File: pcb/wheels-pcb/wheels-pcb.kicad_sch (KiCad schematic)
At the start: 16 parts, among them J1 Motor_1, J2 Motor_2, J3 Motor_3, J4 Motor_4, J5 Conn_01x03, U1 L293D, U2 L293D, U3 ESP32S_38P

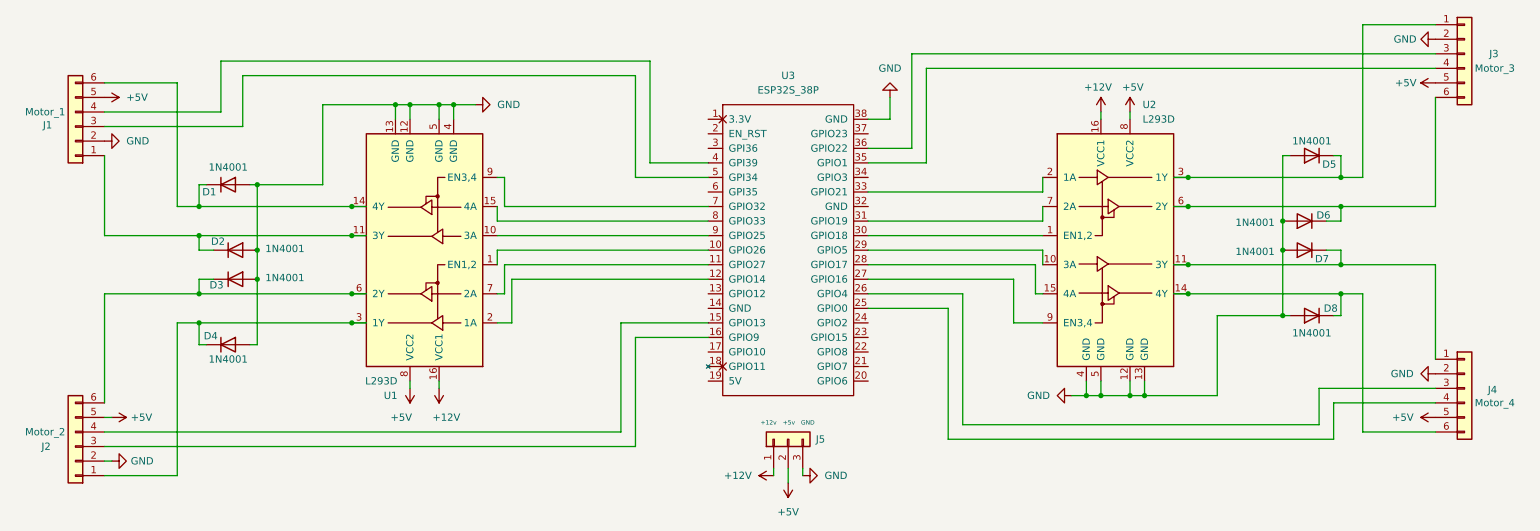
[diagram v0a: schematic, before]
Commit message: pcb correction
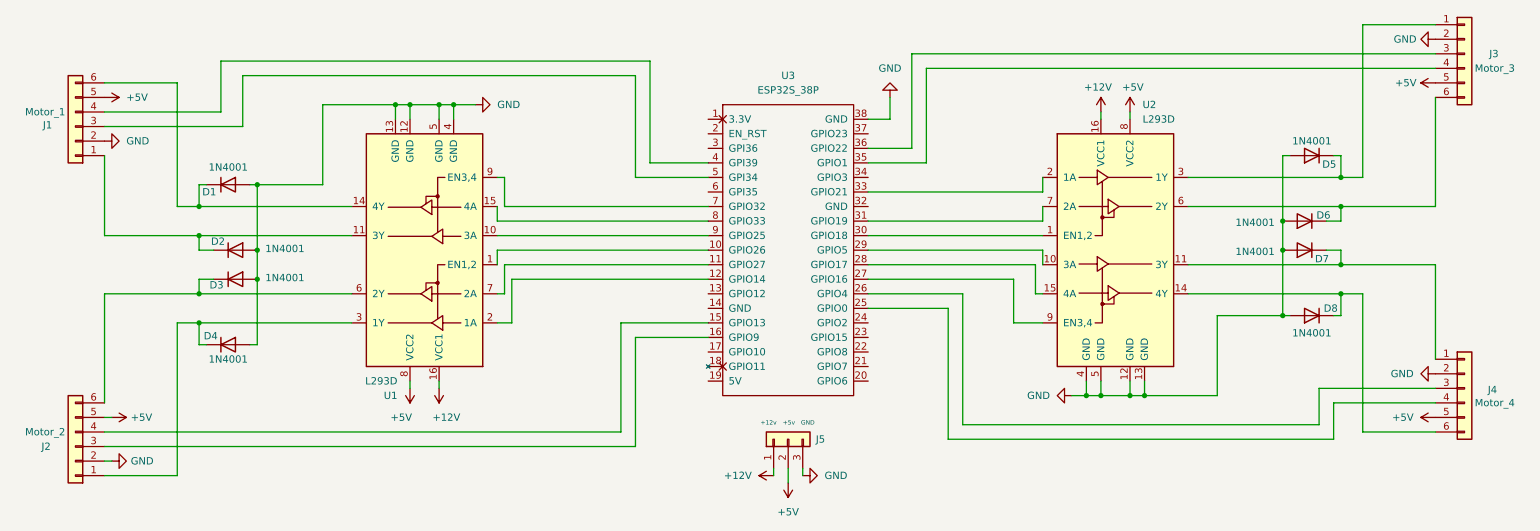
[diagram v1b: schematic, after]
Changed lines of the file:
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@@
-	)
-	(junction
-		(at 222.25 82.55)
-		(diameter 0)
-		(color 0 0 0 0)
 	)
 	(junction
@@
 	)
 	(junction
-		(at 222.25 97.79)
-		(diameter 0)
-		(color 0 0 0 0)
-	)
-	(junction
-		(at 76.2 107.95)
-		(diameter 0)
-		(color 0 0 0 0)
-	)
-	(junction
 		(at 86.36 69.85)
 		(diameter 0)
@@
 	)
 	(junction
-		(at 222.25 102.87)
-		(diameter 0)
-		(color 0 0 0 0)
-	)
-	(junction
-		(at 76.2 92.71)
-		(diameter 0)
-		(color 0 0 0 0)
-	)
-	(junction
 		(at 238.76 95.25)
-		(diameter 0)
-		(color 0 0 0 0)
-	)
-	(junction
-		(at 222.25 87.63)
-		(diameter 0)
-		(color 0 0 0 0)
-	)
-	(junction
-		(at 76.2 102.87)
 		(diameter 0)
 		(color 0 0 0 0)
@@
 	)
 	(junction
-		(at 76.2 87.63)
-		(diameter 0)
-		(color 0 0 0 0)
-	)
-	(junction
 		(at 204.47 120.65)
 		(diameter 0)
@@
 	(wire
 		(pts
-			(xy 78.74 87.63) (xy 76.2 87.63)
-		)
-		(stroke
-			(width 0)
-			(type default)
-		)
-	)
-	(wire
-		(pts
 			(xy 212.09 118.11) (xy 212.09 120.65)
 		)
@@
 	(wire
 		(pts
-			(xy 78.74 107.95) (xy 76.2 107.95)
-		)
-		(stroke
-			(width 0)
-			(type default)
-		)
-	)
-	(wire
-		(pts
 			(xy 248.92 97.79) (xy 265.43 97.79)
 		)
@@
 	(wire
 		(pts
-			(xy 78.74 92.71) (xy 76.2 92.71)
-		)
-		(stroke
-			(width 0)
-			(type default)
-		)
-	)
-	(wire
-		(pts
 			(xy 247.65 106.68) (xy 248.92 106.68)
 		)
@@
 	(wire
 		(pts
-			(xy 219.71 102.87) (xy 222.25 102.87)
-		)
-		(stroke
-			(width 0)
-			(type default)
-		)
-	)
-	(wire
-		(pts
 			(xy 173.99 60.96) (xy 173.99 77.47)
 		)
@@
 	(wire
 		(pts
-			(xy 219.71 82.55) (xy 222.25 82.55)
-		)
-		(stroke
-			(width 0)
-			(type default)
-		)
-	)
-	(wire
-		(pts
 			(xy 182.88 125.73) (xy 245.11 125.73)
 		)
@@
 	(wire
 		(pts
-			(xy 219.71 97.79) (xy 222.25 97.79)
-		)
-		(stroke
-			(width 0)
-			(type default)
-		)
-	)
-	(wire
-		(pts
 			(xy 196.85 97.79) (xy 196.85 95.25)
 		)
@@
 	(wire
 		(pts
-			(xy 219.71 87.63) (xy 222.25 87.63)
-		)
-		(stroke
-			(width 0)
-			(type default)
-		)
-	)
-	(wire
-		(pts
 			(xy 195.58 97.79) (xy 166.37 97.79)
 		)
@@
 		)
 		(stroke
-			(width 0)
-			(type default)
-		)
-	)
-	(wire
-		(pts
-			(xy 78.74 102.87) (xy 76.2 102.87)
-		)
-		(stroke
